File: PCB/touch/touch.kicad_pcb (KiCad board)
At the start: 2 copper layers, 54 x 54 mm, 1 part, among them T1 3Touch

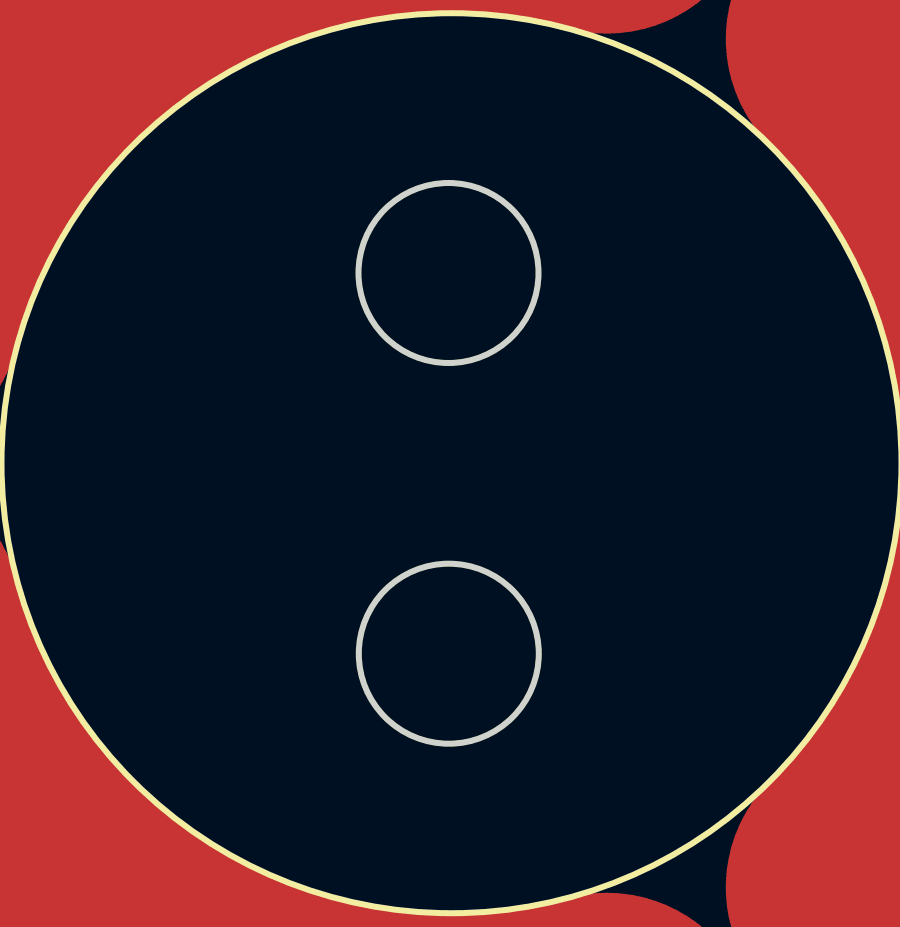
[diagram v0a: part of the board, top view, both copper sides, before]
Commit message: v1.0
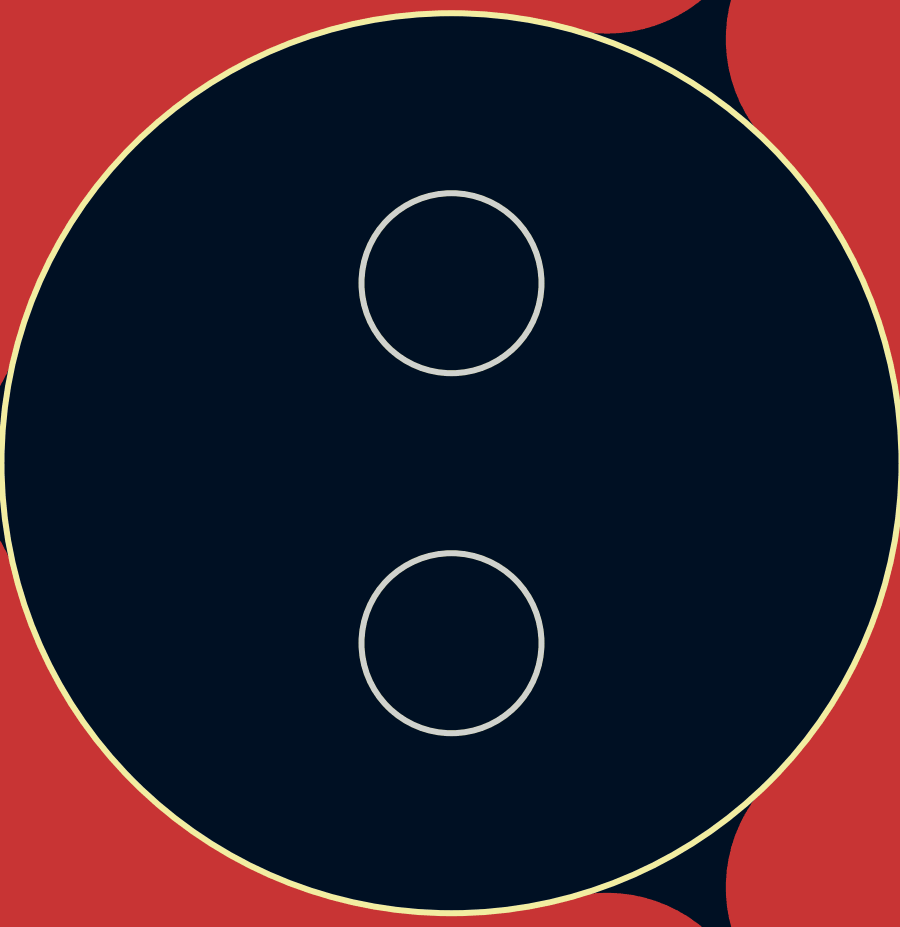
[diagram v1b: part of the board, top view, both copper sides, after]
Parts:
- added G***: LOGO, fsr:FSR_Logo_Small, B.Cu at (-16.8, -0.25)
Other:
- outline, holes or cut-outs redrawn
- board text added: "3-Touch_v1.0"
- board text removed: "3-Touch_v0.1"
